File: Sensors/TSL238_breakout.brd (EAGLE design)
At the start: 27.6 x 17.8 mm, 4 parts

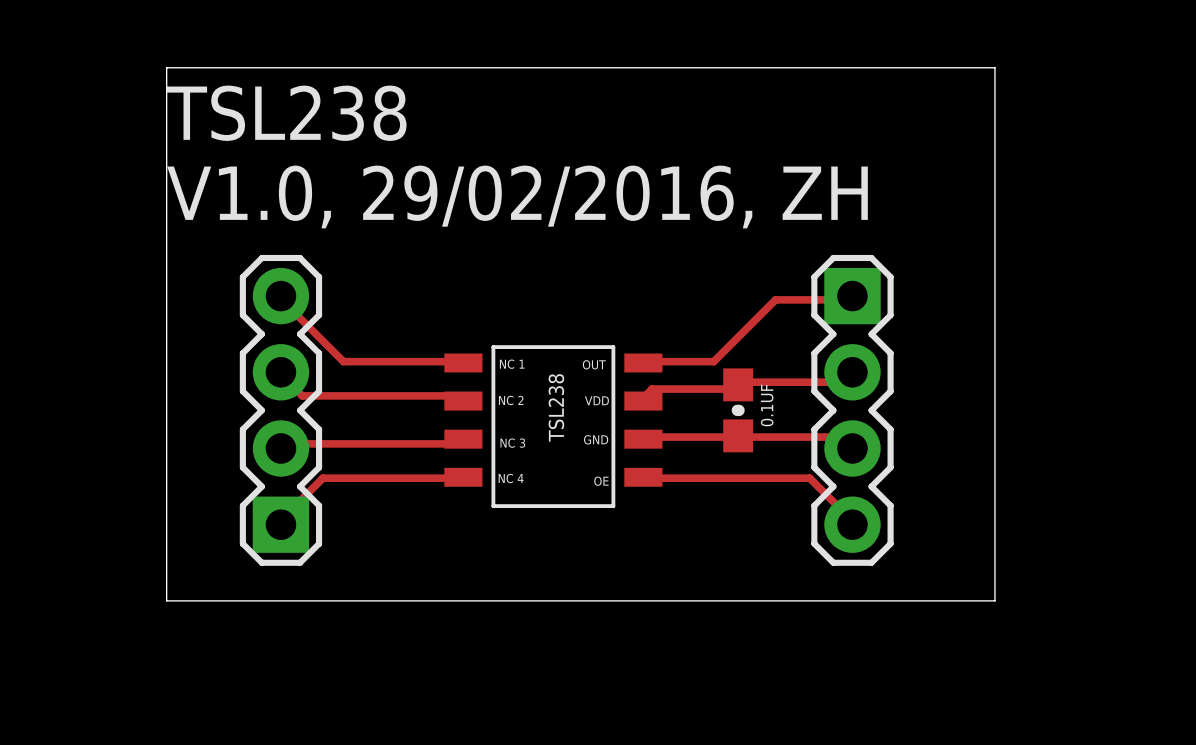
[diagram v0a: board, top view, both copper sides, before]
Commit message: updated tsl238
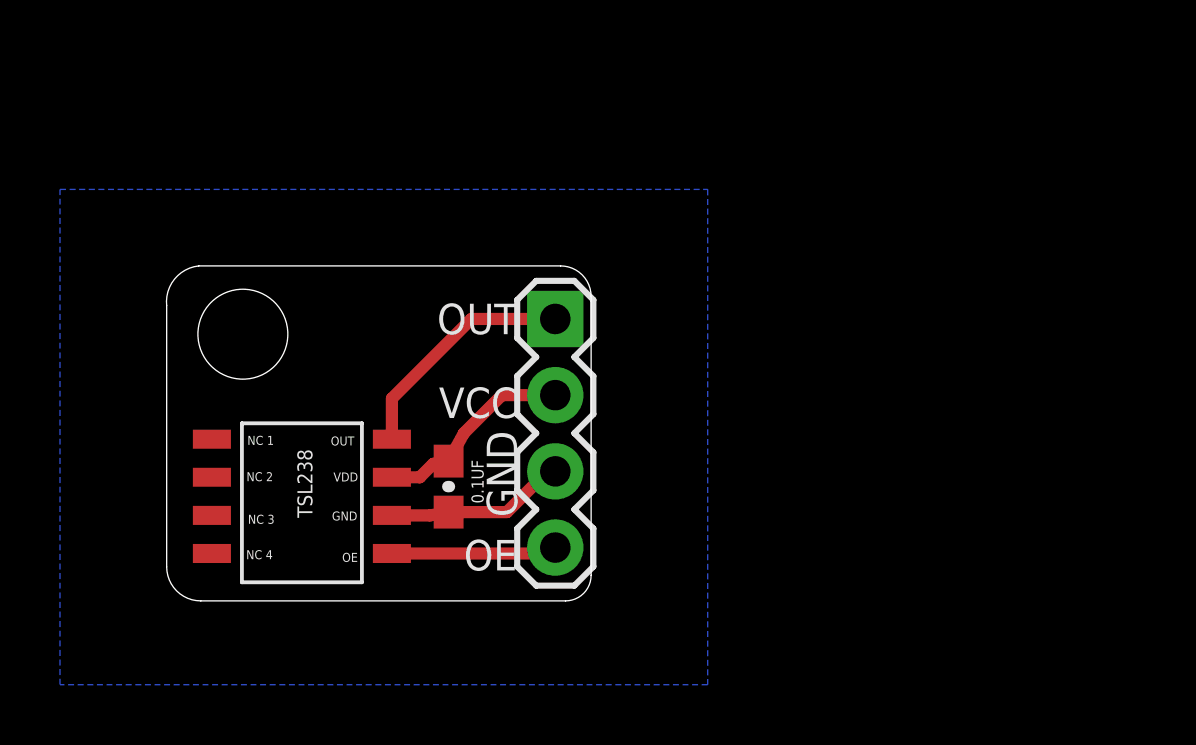
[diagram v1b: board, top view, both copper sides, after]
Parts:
- removed J2: (no value), SparkFun-Connectors:1X04
- moved 0.1UF 9.98 mm to (9.40, 3.81)
- moved J1 9.94 mm to (13.0, 9.40)
- moved U$1 8.76 mm to (4.32, 5.08)
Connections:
- net N$5 renamed OE
- net N$6 renamed VCC
- net N$8 renamed OUT
- net N$9 renamed GND
- removed net N$1: J2.1, U$1.NC4
- removed net N$2: J2.2, U$1.NC3
- removed net N$3: J2.3, U$1.NC2
- removed net N$4: J2.4, U$1.NC1
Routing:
- net N$4: track 7.05 -> 0.00 mm
- net N$1: track 6.81 -> 0.00 mm
- net N$3: track 6.54 -> 0.00 mm
- net N$2: track 6.29 -> 0.00 mm
- net OE: track 7.68 -> 5.53 mm
- net GND: track 7.22 -> 6.02 mm
- net VCC: track 7.44 -> 6.72 mm
- added copper zone on layer 16, net GND
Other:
- board size 27.6 x 17.8 mm -> 14.2 x 11.2 mm
- board text added: "GND"
- board text added: "OE"
- board text added: "OUT"
- board text added: "TSL238 Breakout Board"
- board text added: "VCC"
- board text removed: "TSL238 V1.0, 29/02/2016, ZH"
